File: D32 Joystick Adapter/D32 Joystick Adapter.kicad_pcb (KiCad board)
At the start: 2 copper layers, 30.5 x 31.8 mm, 6 parts, among them J1 MSX, J2 Mega Drive, U1 74HCT04

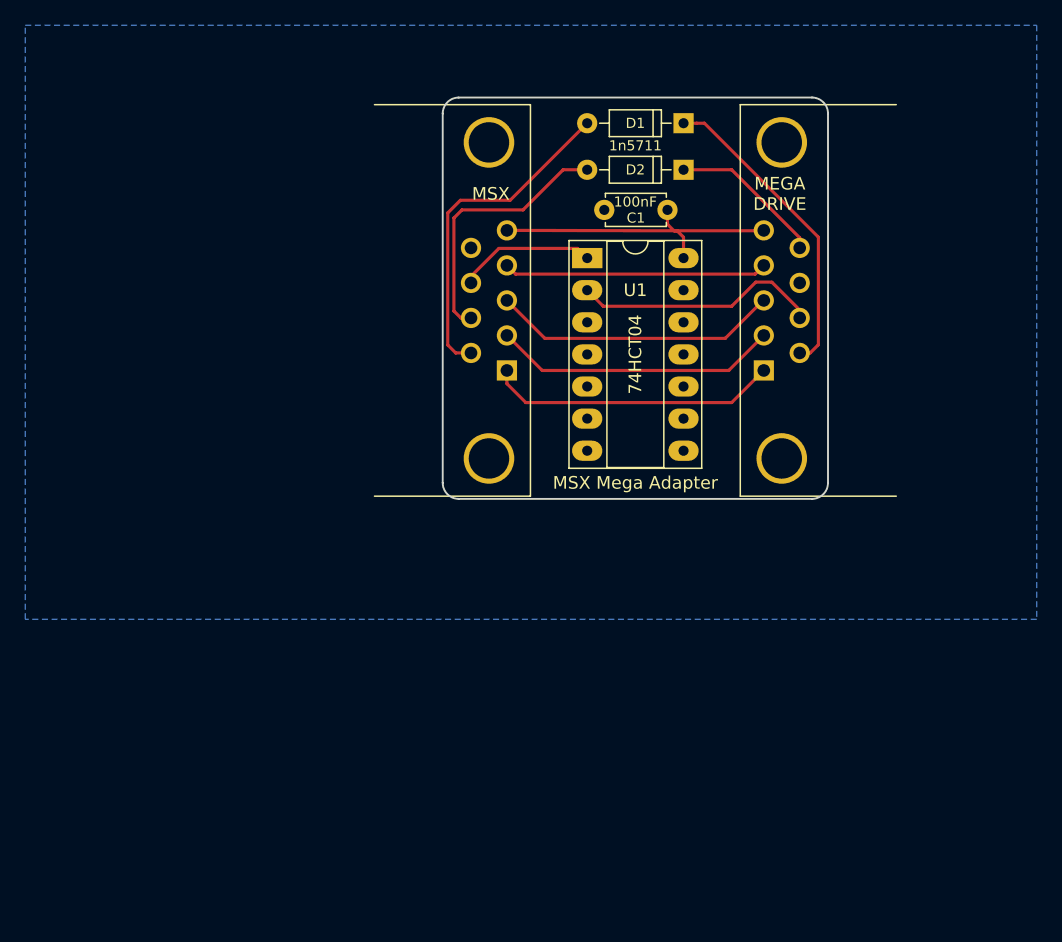
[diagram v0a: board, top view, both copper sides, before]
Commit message: Layout done
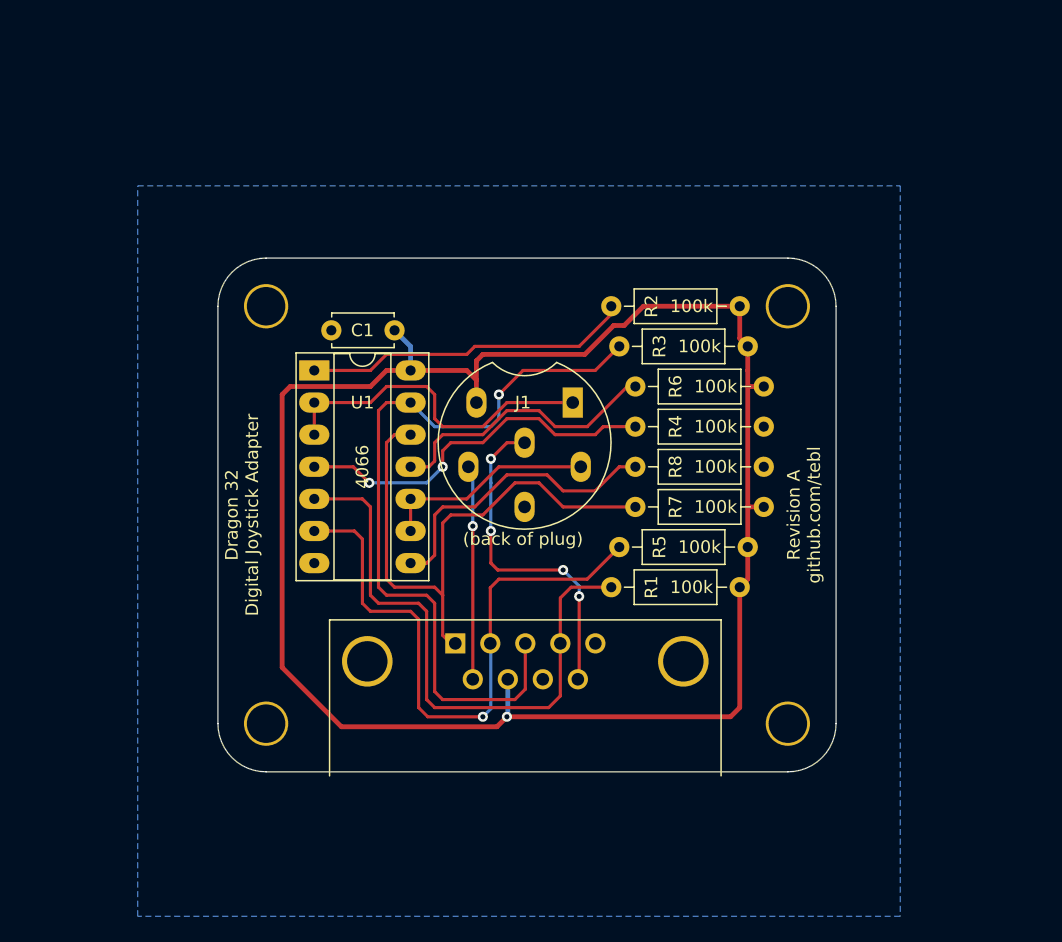
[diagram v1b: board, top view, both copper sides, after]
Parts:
- removed D1, D2: 1n5711, Diodes_THT:D_DO-35_SOD27_P7.62mm_Horizontal
- added M1: Mounting, mounting:M3_pin, F.Cu at (102.2, 108.6)
- added M2: Mounting, mounting:M3_pin, F.Cu at (143.5, 108.6)
- added M3: Mounting, mounting:M3_pin, F.Cu at (143.5, 75.6)
- added M4: Mounting, mounting:M3_pin, F.Cu at (102.2, 75.6)
- added R1: 100k, Resistor_THT:R_Axial_DIN0207_L6.3mm_D2.5mm_P10.16mm_Horizontal, F.Cu at (129.5, 97.8)
- added R2: 100k, Resistor_THT:R_Axial_DIN0207_L6.3mm_D2.5mm_P10.16mm_Horizontal, F.Cu at (129.5, 75.6)
- added R3: 100k, Resistor_THT:R_Axial_DIN0207_L6.3mm_D2.5mm_P10.16mm_Horizontal, F.Cu at (130.2, 78.7)
- added R4: 100k, Resistor_THT:R_Axial_DIN0207_L6.3mm_D2.5mm_P10.16mm_Horizontal, F.Cu at (141.6, 85.1)
- added R5: 100k, Resistor_THT:R_Axial_DIN0207_L6.3mm_D2.5mm_P10.16mm_Horizontal, F.Cu at (130.2, 94.6)
- added R6: 100k, Resistor_THT:R_Axial_DIN0207_L6.3mm_D2.5mm_P10.16mm_Horizontal, F.Cu at (131.4, 81.9)
- added R7: 100k, Resistor_THT:R_Axial_DIN0207_L6.3mm_D2.5mm_P10.16mm_Horizontal, F.Cu at (131.4, 91.4)
- added R8: 100k, Resistor_THT:R_Axial_DIN0207_L6.3mm_D2.5mm_P10.16mm_Horizontal, F.Cu at (141.6, 88.3)
- C1: footprint Capacitors_THT:C_Disc_D4.7mm_W2.5mm_P5.00mm -> Capacitor_THT:C_Disc_D4.7mm_W2.5mm_P5.00mm
- J1: value MSX -> Dragon 32; footprint RND:DSUB-9_Female_Horizontal_P2.77x2.84mm_EdgePinOffset7.70mm_Housed_MountingHolesOffset9.12mm -> D32_Wirepads:OUTPUT_ZIP
- J2: value Mega Drive -> Joystick
- U1: value 74HCT04 -> 4066; footprint Housings_DIP:DIP-14_W7.62mm_Socket_LongPads -> Package_DIP:DIP-14_W7.62mm_Socket_LongPads
- moved J2 32.6 mm to (117.2, 102.2), turned to 0 degrees
- moved C1 23.6 mm to (112.4, 77.5)
- moved U1 23.3 mm to (106.0, 80.6)
- moved J1 5.88 mm to (122.7, 86.4), turned to 90 degrees
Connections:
- J1 pad 1: UP -> POT_X
- J1 pad 2: DOWN -> POT_Y
- J1 pad 3: LEFT -> GND
- J1 pad 4: RIGHT -> FIRE1
- J1 pad 6: TRIGGER1 -> FIRE2
- J2 pad 5: VCC -> Net-(J2-Pad5)
- J2 pad 6: Net-(D1-Pad1) -> FIRE1
- J2 pad 7: Net-(J2-Pad7) -> VCC
- J2 pad 9: Net-(D2-Pad1) -> FIRE2
- U1 pad 1: OUT -> Net-(R2-Pad1)
- U1 pad 10: (no net) -> POT_Y
- U1 pad 11: GND -> Net-(R6-Pad1)
- U1 pad 12: (no net) -> UP
- U1 pad 13: GND -> LEFT
- U1 pad 2: Net-(J2-Pad7) -> POT_X
- U1 pad 3: GND -> POT_X
- U1 pad 4: (no net) -> Net-(R4-Pad2)
- U1 pad 5: GND -> RIGHT
- U1 pad 6: (no net) -> DOWN
- U1 pad 8: (no net) -> Net-(R8-Pad2)
- U1 pad 9: GND -> POT_Y
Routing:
- net VCC: track 24.7 -> 144.3 mm, vias 0 -> 1
- net LEFT: track 22.8 -> 61.2 mm, vias 0 -> 1
- net Net-(R4-Pad2): track 0.00 -> 29.6 mm, vias 0 -> 2
- net POT_X: track 0.00 -> 26.7 mm
- net FIRE2: track 0.00 -> 26.6 mm, vias 0 -> 4
- net TRIGGER1: track 26.5 -> 0.00 mm
- net RIGHT: track 20.9 -> 47.0 mm
- net Net-(R2-Pad1): track 0.00 -> 26.0 mm
- net DOWN: track 22.6 -> 48.5 mm, vias 0 -> 1
- net Net-(D1-Pad1): track 24.7 -> 0.00 mm
- net Net-(R8-Pad2): track 0.00 -> 23.8 mm
- net UP: track 23.0 -> 45.4 mm
- net Net-(R6-Pad1): track 0.00 -> 22.3 mm
- net TRIGGER2: track 21.1 -> 0.00 mm
- net Net-(J2-Pad7): track 19.7 -> 0.00 mm
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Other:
- board size 30.5 x 31.8 mm -> 48.9 x 40.6 mm
- net class Default: via_dia 0.6 -> 0.8
- net class PWR added: clearance 0.2, trace_width 0.381, via_dia 0.8, via_drill 0.4
- net class Power removed
- rule pad_to_mask_clearance: 0.2 -> 0
- board text added: "(back of plug)"
- board text added: "Dragon 32 Digital Joystick Adapter"
- board text added: "Revision A github.com/tebl"
- board text removed: "Licensed under CERN OHL v.1.2"
- board text removed: "MEGA DRIVE"
- board text removed: "MSX"
- board text removed: "MSX Mega Adapter"
- board text removed: "github.com/tebl"
